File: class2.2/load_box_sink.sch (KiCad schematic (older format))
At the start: 38 parts, among them J2 Screw_Terminal_1x02, J3 Screw_Terminal_1x02, J6 CONN_01X02, Q1 Q_NMOS_GDS, Q2 Q_NMOS_GDS, Q3 Q_NMOS_GDS, U1 LM324, U2 INA128

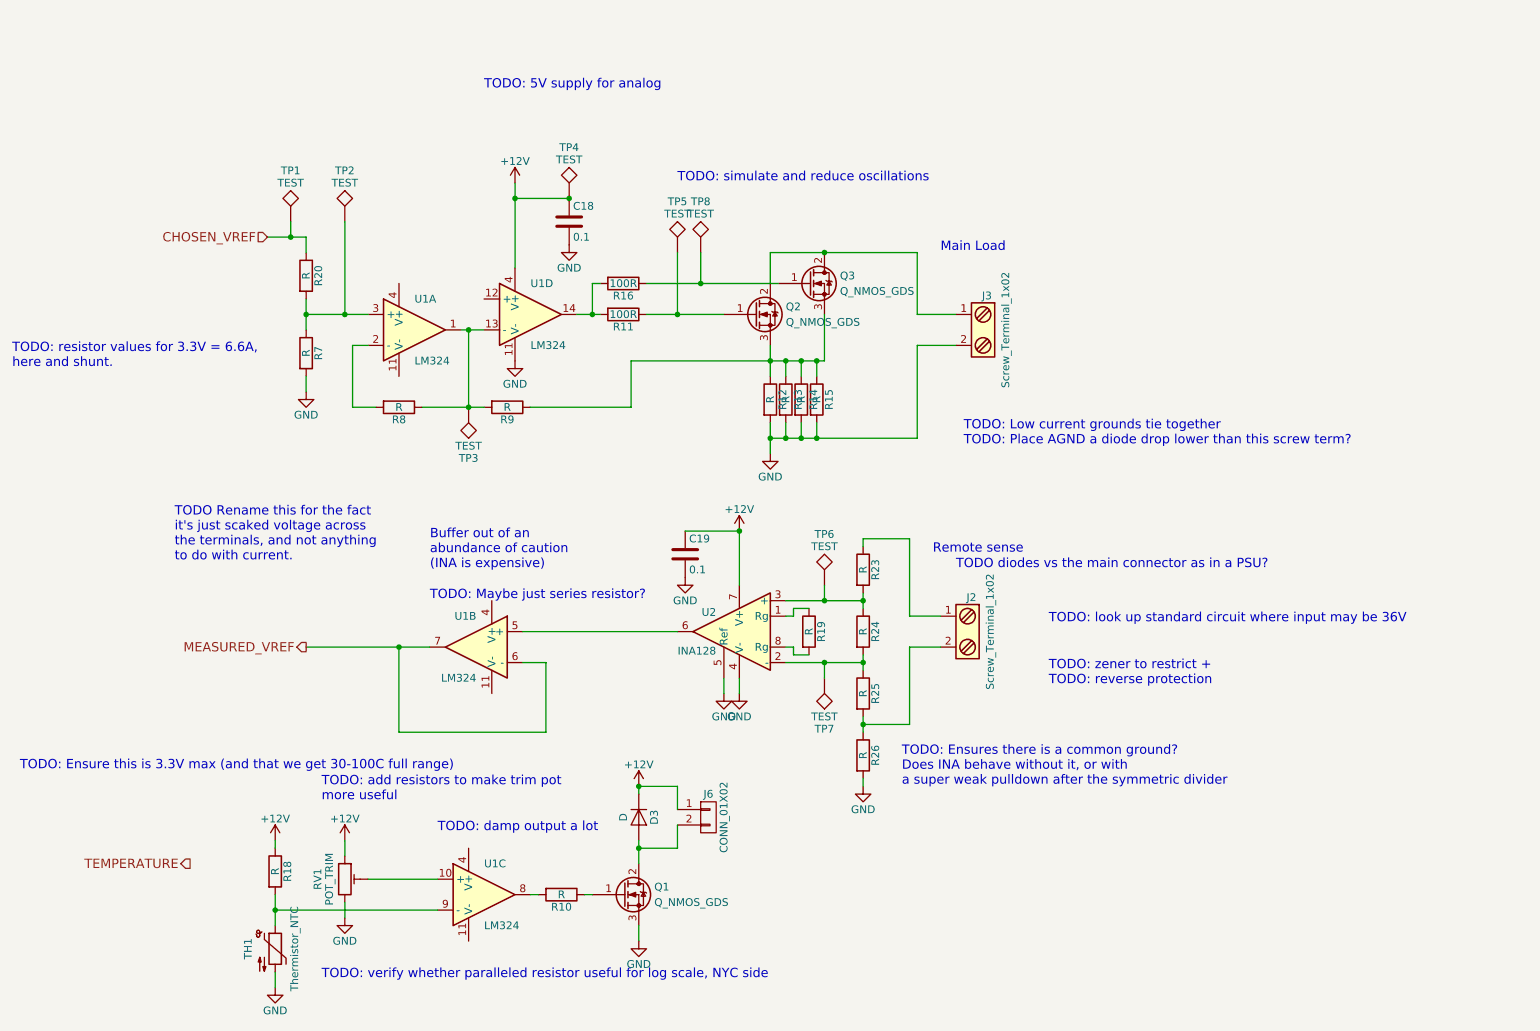
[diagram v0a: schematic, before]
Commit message: Checkpoint with NHD, 3.3v, and layout
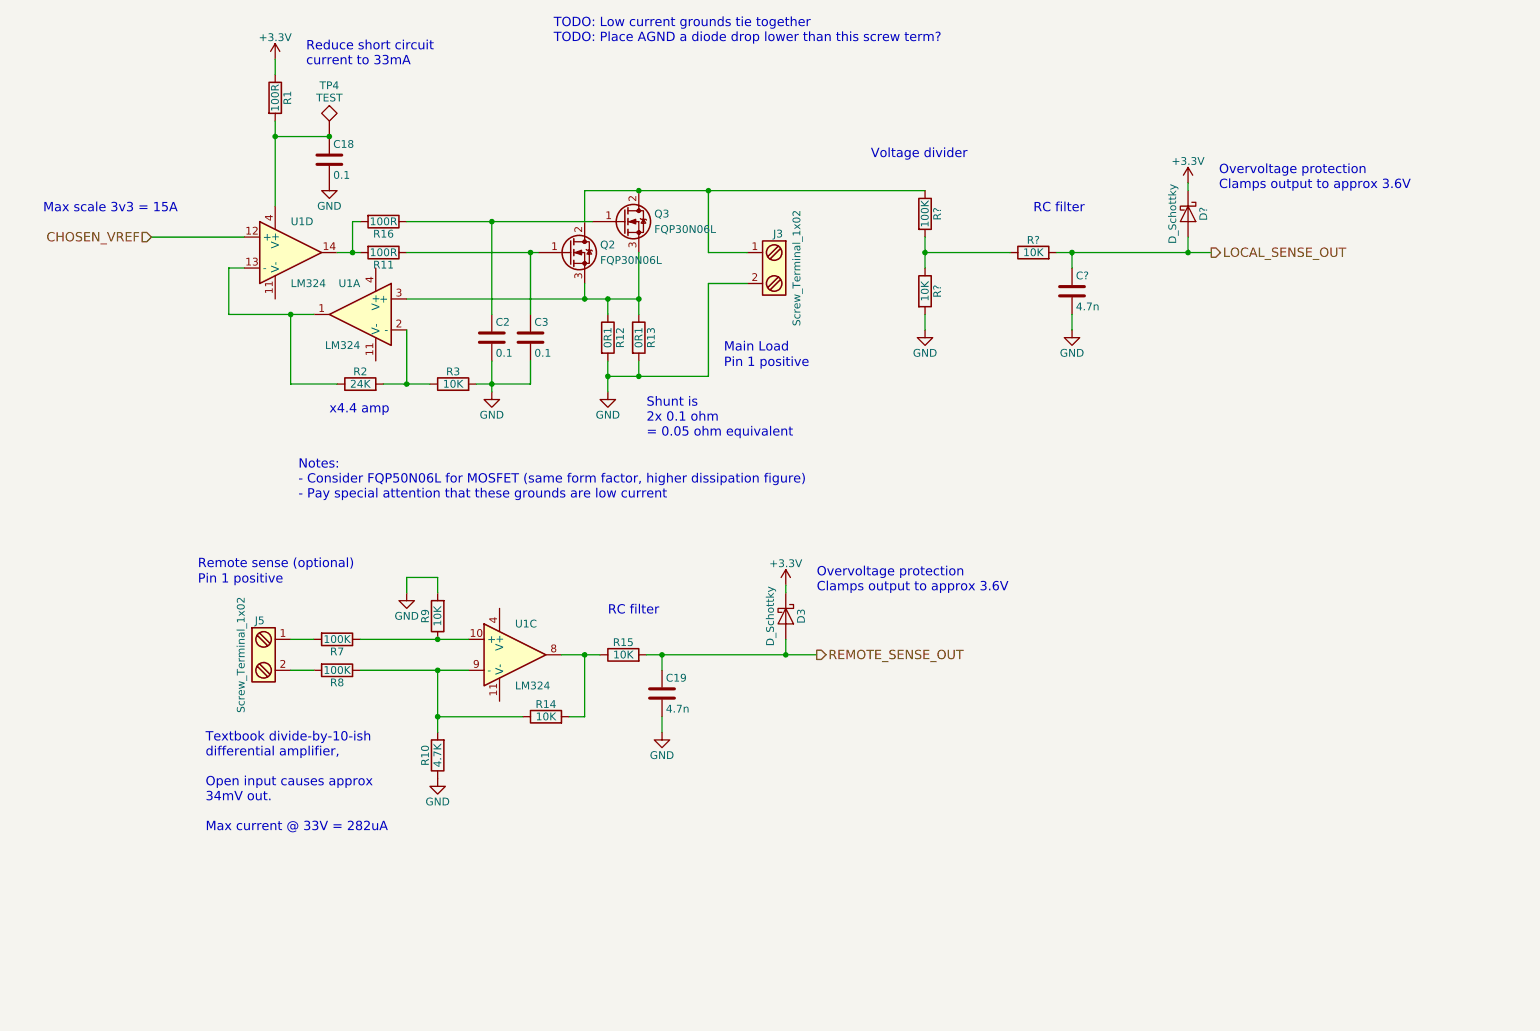
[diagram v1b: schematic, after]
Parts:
- removed D3: D, Diodes_SMD:D_SOD-123, symbol D
- removed J2: Screw_Terminal_1x02, Connectors_Terminal_Blocks:TerminalBlock_Pheonix_MKDS1.5-2pol, symbol Screw_Terminal_1x02
- removed J6: CONN_01X02, Connectors_JST:JST_XH_B02B-XH-A_02x2.50mm_Straight, symbol CONN_01X02
- removed Q1: Q_NMOS_GDS, TO_SOT_Packages_SMD:SOT-23, symbol Q_NMOS_GDS
- removed R18, R19, R20, R23, R24, R25, R26: R, Resistors_SMD:R_0603, symbol R
- removed RV1: POT_TRIM, Potentiometers:Potentiometer_Trimmer_Bourns_3214G, symbol POT_TRIM
- removed TH1: Thermistor_NTC, Connectors_JST:JST_XH_B02B-XH-A_02x2.50mm_Straight, symbol Thermistor_NTC
- removed TP1, TP2, TP3, TP5, TP6, TP7, TP8: TEST, Measurement_Points:Test_Point, symbol TEST
- removed unit 2 of U1
- removed U2: INA128, Housings_SOIC:SOIC-8_3.9x4.9mm_Pitch1.27mm, symbol INA128
- added C2, C3: 0.1, Capacitors_SMD:C_0603, symbol C
- added C?: 4.7n, Capacitors_SMD:C_0603, symbol C
- added D3, D?: D_Schottky, Diodes_SMD:D_SOD-123, symbol D_Schottky
- added J5: Screw_Terminal_1x02, Connectors_Terminal_Blocks:TerminalBlock_Pheonix_MKDS1.5-2pol, symbol Screw_Terminal_1x02
- added R1: 100R, Resistors_SMD:R_0603, symbol R
- added R2: 24K, Resistors_SMD:R_0603, symbol R
- added R3, R? (x2): 10K, Resistors_SMD:R_0603, symbol R
- added R?: 100K, Resistors_SMD:R_0603, symbol R
- C19: value 0.1 -> 4.7n
- Q2, Q3: value Q_NMOS_GDS -> FQP30N06L
- R10: value R -> 4.7K
- R12, R13: value R -> 0R1; footprint Resistors_THT:R_Axial_DIN0516_L15.5mm_D5.0mm_P20.32mm_Horizontal -> Resistors_SMD:R_2512
- R14, R15: value R -> 10K; footprint Resistors_THT:R_Axial_DIN0516_L15.5mm_D5.0mm_P20.32mm_Horizontal -> Resistors_SMD:R_0603
- R7, R8: value R -> 100K
- R9: value R -> 10K
- TP4: footprint Measurement_Points:Test_Point -> Measurement_Points:Measurement_Point_Round-TH_Big
- U1: footprint Housings_SOIC:SOIC-14_3.9x8.7mm_Pitch1.27mm -> (none)
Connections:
- net CHOSEN_VREF: now also U1.12 (+)
- net GND: now also R10.1, R9.2, C2.2, C3.2, C?.2, R3.2, R?.2; no longer R14.2, R15.2, R7.2, U1.11 (V-)
- net at Q2.3 (S), Q3.3 (S), R12.1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: now also U1.3 (+); no longer R14.1, R15.1, R9.1
- net at U1.1, U1.13 (-): now also R2.1; no longer R8.1, R9.2
- net at U1.2 (-): now also R2.2, R3.1; no longer R8.2
- net at R7.1: now also R9.1, U1.10 (+); no longer U1.3 (+)
- net at U1.8: now also R14.2, R15.1; no longer R10.2
- net at U1.9 (-): now also R10.2, R14.1, R8.1
- net at J3.1, Q2.2 (D), Q3.2 (D): now also R?.1
- net at Q2.1 (G), R11.1: now also C3.1
- net at Q3.1 (G), R16.1: now also C2.1
- net +12V: no longer names the net of C18.1, TP4.1, U1.4 (V+)
- net +12V: now also R1.2; no longer C19.1
- new net: J5.1, R7.2
- new net: J5.2, R8.2
- new net: R?.1, R?.1, R?.2
- new net +3V3: D3.1 (K), D?.1 (K), R1.1
- new net LOCAL_SENSE_OUT: C?.1, D?.2 (A), R?.2
- new net REMOTE_SENSE_OUT: C19.1, D3.2 (A), R15.2
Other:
- note added: "Max scale 3v3 = 15A"
- note added: "Notes:\n- Consider FQP50N06L for MOSFET (same form factor, higher dissipation figure)\n- Pay special attention that these grounds are low current"
- note added: "Overvoltage protection\nClamps output to approx 3.6V"
- note added: "Pin 1 positive"
- note added: "RC filter"
- note added: "Reduce short circuit\ncurrent to 33mA"
- note added: "Remote sense (optional)"
- note added: "Shunt is\n2x 0.1 ohm\n= 0.05 ohm equivalent"
- note added: "Textbook divide-by-10-ish\ndifferential amplifier,\n\nOpen input causes approx\n34mV out.\n\nMax current @ 33V = 282uA"
- note added: "Voltage divider"
- note added: "x4.4 amp"
- note removed: "Buffer out of an\nabundance of caution\n(INA is expensive)"
- note removed: "Remote sense"
- note removed: "TODO Rename this for the fact\nit's just scaked voltage across\nthe terminals, and not anything\nto do with current."
- note removed: "TODO diodes vs the main connector as in a PSU?"
- note removed: "TODO: 5V supply for analog"
- note removed: "TODO: Ensure this is 3.3V max (and that we get 30-100C full range)"
- note removed: "TODO: Ensures there is a common ground?\nDoes INA behave without it, or with\na super weak pulldown after the symmetric divider"
- note removed: "TODO: Maybe just series resistor?"
- note removed: "TODO: add resistors to make trim pot\nmore useful"
- note removed: "TODO: damp output a lot"
- note removed: "TODO: look up standard circuit where input may be 36V"
- note removed: "TODO: resistor values for 3.3V = 6.6A,\nhere and shunt."
- note removed: "TODO: simulate and reduce oscillations"
- note removed: "TODO: verify whether paralleled resistor useful for log scale, NYC side"
- note removed: "TODO: zener to restrict +\nTODO: reverse protection"
- moved on the sheet: C18, J3, Q2, Q3, R11, R12, R13, R16, TP4, U1A, U1D
